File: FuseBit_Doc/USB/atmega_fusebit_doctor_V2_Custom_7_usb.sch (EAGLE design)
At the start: 73 parts, among them IC1 7805, IC10 MEGA8/88/168..., IC11 MEGA8-AI, IC12 FT232RL, IC14 TINY2313, IC15 MEGA16, IC16 MEGA128-A, IC17 MEGA8/88/168..., IC2 ATMEGA8-DOC, IC3 MEGA16/32/644..., IC4 MEGA8/88/168..., IC5 AT90S2313/TINY2313, IC8 AT90S8515PDIL40_OCT, IC9 TINY26, T1 BC857, T2 BC847, T3 BC557

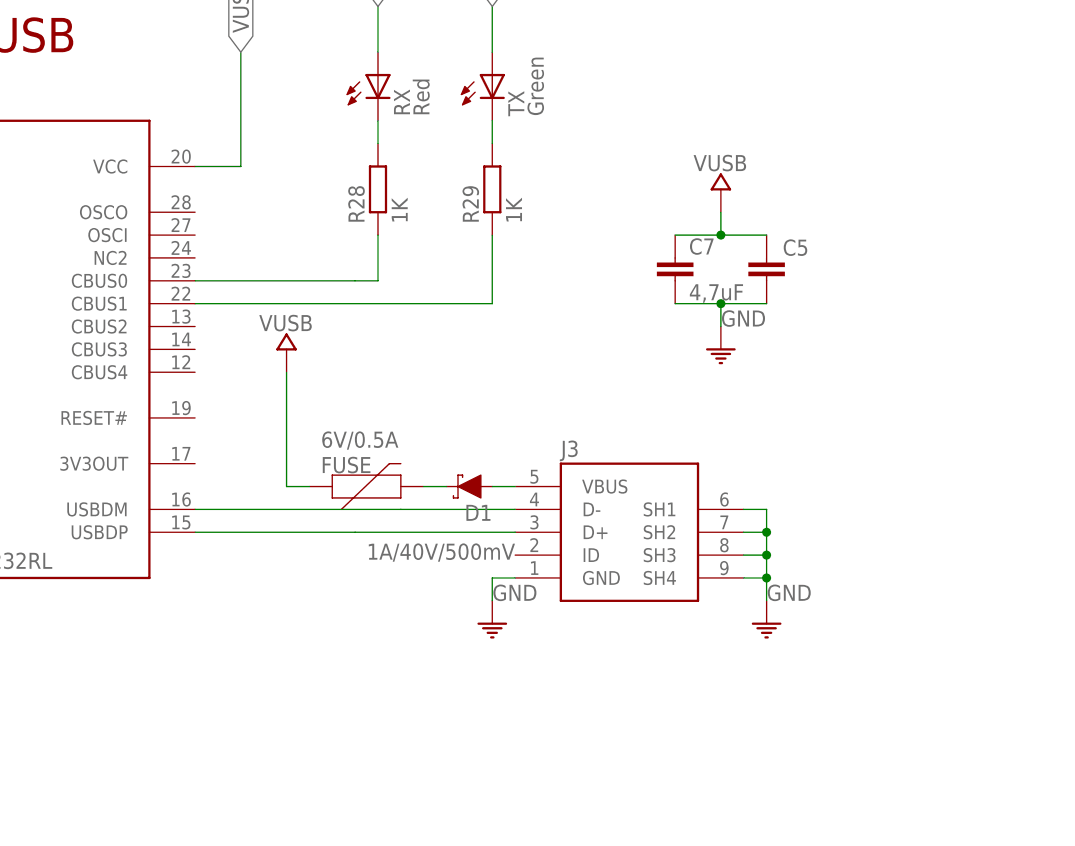
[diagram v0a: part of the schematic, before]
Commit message: FT232_update
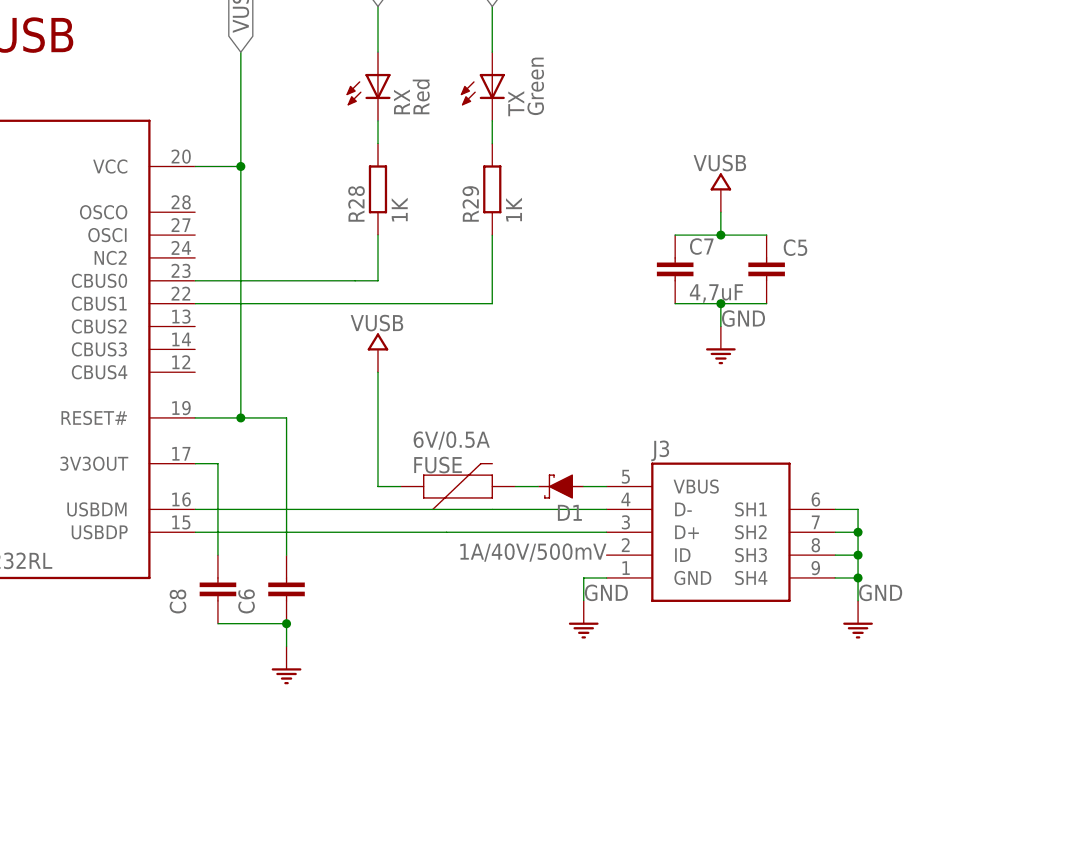
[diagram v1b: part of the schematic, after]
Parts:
- added C6, C8: 100nF, resistor@1:C-EUC0805
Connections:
- new net COM: C6.1, C8.1
- new net N$3: C8.2, IC12.3V3OUT
- net VUSB: now also C6.2, IC12.RESET#
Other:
- moved on the sheet: D1, FUSE, J3
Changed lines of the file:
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@@
 <?xml version="1.0" encoding="utf-8"?>
 <!DOCTYPE eagle SYSTEM "eagle.dtd">
-<eagle version="7.6.0">
+<eagle version="8.5.1">
 <drawing>
 <settings>
 <setting alwaysvectorfont="no"/>
+<setting keepoldvectorfont="yes"/>
 <setting verticaltext="up"/>
 </settings>
@@
 <part name="U$4" library="MyPOW" deviceset="VUSB" device=""/>
 <part name="D1" library="SparkFun-DiscreteSemi" deviceset="DIODE-SCHOTTKY" device="-SS14" value="1A/40V/500mV"/>
+<part name="C6" library="resistor@1" deviceset="C-EU" device="C0805" value="100nF"/>
+<part name="U$1" library="MyPOW" deviceset="COM" device=""/>
+<part name="C8" library="resistor@1" deviceset="C-EU" device="C0805" value="100nF"/>
 </parts>
 <sheets>
@@
 </instance>
 <instance part="U$24" gate="G$1" x="302.26" y="193.04"/>
-<instance part="U$22" gate="G$1" x="350.52" y="220.98"/>
-<instance part="U$29" gate="G$1" x="373.38" y="190.5"/>
-<instance part="U$30" gate="G$1" x="403.86" y="190.5"/>
-<instance part="J3" gate="G$1" x="388.62" y="200.66"/>
+<instance part="U$22" gate="G$1" x="360.68" y="220.98"/>
+<instance part="U$29" gate="G$1" x="383.54" y="190.5"/>
+<instance part="U$30" gate="G$1" x="414.02" y="190.5"/>
+<instance part="J3" gate="G$1" x="398.78" y="200.66"/>
 <instance part="U$51" gate="G$1" x="289.56" y="203.2"/>
 <instance part="RX" gate="G$1" x="360.68" y="251.46"/>
 <instance part="TX" gate="G$1" x="373.38" y="251.46"/>
 <instance part="IC12" gate="G$1" x="322.58" y="220.98"/>
-<instance part="FUSE" gate="G$1" x="358.14" y="205.74" smashed="yes">
-<attribute name="NAME" x="354.33" y="207.2386" size="1.778" layer="95"/>
-<attribute name="VALUE" x="354.33" y="210.058" size="1.778" layer="96"/>
+<instance part="FUSE" gate="G$1" x="368.3" y="205.74" smashed="yes">
+<attribute name="NAME" x="364.49" y="207.2386" size="1.778" layer="95"/>
+<attribute name="VALUE" x="364.49" y="210.058" size="1.778" layer="96"/>
 </instance>
 <instance part="R28" gate="G$1" x="360.68" y="238.76" rot="R90"/>
@@
 <instance part="C7" gate="G$1" x="393.7" y="231.14"/>
 <instance part="U$4" gate="G$1" x="398.78" y="238.76"/>
-<instance part="D1" gate="G$1" x="370.84" y="205.74" smashed="yes" rot="R180">
-<attribute name="NAME" x="373.38" y="203.708" size="1.778" layer="95" font="vector" rot="R180"/>
-<attribute name="VALUE" x="375.92" y="197.612" size="1.778" layer="96" font="vector" rot="R180" align="top-left"/>
+<instance part="D1" gate="G$1" x="381" y="205.74" smashed="yes" rot="R180">
+<attribute name="NAME" x="383.54" y="203.708" size="1.778" layer="95" font="vector" rot="R180"/>
+<attribute name="VALUE" x="386.08" y="197.612" size="1.778" layer="96" font="vector" rot="R180" align="top-left"/>
+</instance>
+<instance part="C6" gate="G$1" x="350.52" y="193.04" smashed="yes" rot="R180">
+<attribute name="NAME" x="346.964" y="191.516" size="1.778" layer="95" rot="R90"/>
+</instance>
+<instance part="U$1" gate="G$1" x="350.52" y="185.42"/>
+<instance part="C8" gate="G$1" x="342.9" y="193.04" smashed="yes" rot="R180">
+<attribute name="NAME" x="339.344" y="191.516" size="1.778" layer="95" rot="R90"/>
 </instance>
 </instances>
@@
 </segment>
 <segment>
-<wire x1="375.92" y1="195.58" x2="373.38" y2="195.58" width="0.1524" layer="91"/>
-<wire x1="373.38" y1="195.58" x2="373.38" y2="193.04" width="0.1524" layer="91"/>
+<wire x1="386.08" y1="195.58" x2="383.54" y2="195.58" width="0.1524" layer="91"/>
+<wire x1="383.54" y1="195.58" x2="383.54" y2="193.04" width="0.1524" layer="91"/>
 <pinref part="U$29" gate="G$1" pin="COM"/>
 <pinref part="J3" gate="G$1" pin="GND"/>
-<label x="373.38" y="193.04" size="1.778" layer="95"/>
+<label x="383.54" y="193.04" size="1.778" layer="95"/>
 </segment>
 <segment>
-<wire x1="403.86" y1="203.2" x2="403.86" y2="200.66" width="0.1524" layer="91"/>
-<wire x1="403.86" y1="200.66" x2="403.86" y2="198.12" width="0.1524" layer="91"/>
-<wire x1="403.86" y1="198.12" x2="403.86" y2="195.58" width="0.1524" layer="91"/>
-<wire x1="403.86" y1="195.58" x2="403.86" y2="193.04" width="0.1524" layer="91"/>
-<wire x1="401.32" y1="200.66" x2="403.86" y2="200.66" width="0.1524" layer="91"/>
-<wire x1="401.32" y1="195.58" x2="403.86" y2="195.58" width="0.1524" layer="91"/>
-<wire x1="401.32" y1="198.12" x2="403.86" y2="198.12" width="0.1524" layer="91"/>
-<wire x1="401.32" y1="203.2" x2="403.86" y2="203.2" width="0.1524" layer="91"/>
+<wire x1="414.02" y1="203.2" x2="414.02" y2="200.66" width="0.1524" layer="91"/>
+<wire x1="414.02" y1="200.66" x2="414.02" y2="198.12" width="0.1524" layer="91"/>
+<wire x1="414.02" y1="198.12" x2="414.02" y2="195.58" width="0.1524" layer="91"/>
+<wire x1="414.02" y1="195.58" x2="414.02" y2="193.04" width="0.1524" layer="91"/>
+<wire x1="411.48" y1="200.66" x2="414.02" y2="200.66" width="0.1524" layer="91"/>
+<wire x1="411.48" y1="195.58" x2="414.02" y2="195.58" width="0.1524" layer="91"/>
+<wire x1="411.48" y1="198.12" x2="414.02" y2="198.12" width="0.1524" layer="91"/>
+<wire x1="411.48" y1="203.2" x2="414.02" y2="203.2" width="0.1524" layer="91"/>
 <pinref part="U$30" gate="G$1" pin="COM"/>
 <pinref part="J3" gate="G$1" pin="SH2"/>
@@
 <pinref part="J3" gate="G$1" pin="SH3"/>
 <pinref part="J3" gate="G$1" pin="SH1"/>
-<junction x="403.86" y="200.66"/>
-<junction x="403.86" y="198.12"/>
-<junction x="403.86" y="195.58"/>
-<label x="403.86" y="193.04" size="1.778" layer="95"/>
+<junction x="414.02" y="200.66"/>
+<junction x="414.02" y="198.12"/>
+<junction x="414.02" y="195.58"/>
+<label x="414.02" y="193.04" size="1.778" layer="95"/>
 </segment>
 <segment>
@@
 <net name="VUSB" class="1">
 <segment>
-<wire x1="350.52" y1="205.74" x2="350.52" y2="218.44" width="0.1524" layer="91"/>
+<wire x1="360.68" y1="205.74" x2="360.68" y2="218.44" width="0.1524" layer="91"/>
 <pinref part="U$22" gate="G$1" pin="VUSB"/>
 <pinref part="FUSE" gate="G$1" pin="1"/>
-<wire x1="350.52" y1="205.74" x2="353.06" y2="205.74" width="0.1524" layer="91"/>
+<wire x1="360.68" y1="205.74" x2="363.22" y2="205.74" width="0.1524" layer="91"/>
 </segment>
 <segment>
@@
 <wire x1="345.44" y1="241.3" x2="345.44" y2="254" width="0.1524" layer="91"/>
 <label x="345.44" y="254" size="1.778" layer="95" rot="R90" xref="yes"/>
+<wire x1="345.44" y1="241.3" x2="345.44" y2="213.36" width="0.1524" layer="91"/>
+<junction x="345.44" y="241.3"/>
+<pinref part="IC12" gate="G$1" pin="RESET#"/>
+<wire x1="345.44" y1="213.36" x2="340.36" y2="213.36" width="0.1524" layer="91"/>
+<pinref part="C6" gate="G$1" pin="2"/>
+<wire x1="345.44" y1="213.36" x2="350.52" y2="213.36" width="0.1524" layer="91"/>
+<wire x1="350.52" y1="213.36" x2="350.52" y2="198.12" width="0.1524" layer="91"/>
+<junction x="345.44" y="213.36"/>
 </segment>
 <segment>
@@
 <net name="N$44" class="0">
 <segment>
-<wire x1="340.36" y1="200.66" x2="358.14" y2="200.66" width="0.1524" layer="91"/>
+<wire x1="340.36" y1="200.66" x2="368.3" y2="200.66" width="0.1524" layer="91"/>
 <pinref part="J3" gate="G$1" pin="D+"/>
 <pinref part="IC12" gate="G$1" pin="USBDP"/>
-<wire x1="358.14" y1="200.66" x2="375.92" y2="200.66" width="0.1524" layer="91"/>
+<wire x1="368.3" y1="200.66" x2="386.08" y2="200.66" width="0.1524" layer="91"/>
 </segment>
 </net>
 <net name="N$45" class="0">
 <segment>
-<wire x1="340.36" y1="203.2" x2="363.22" y2="203.2" width="0.1524" layer="91"/>
+<wire x1="340.36" y1="203.2" x2="373.38" y2="203.2" width="0.1524" layer="91"/>
 <pinref part="J3" gate="G$1" pin="D-"/>
 <pinref part="IC12" gate="G$1" pin="USBDM"/>
-<wire x1="363.22" y1="203.2" x2="375.92" y2="203.2" width="0.1524" layer="91"/>
+<wire x1="373.38" y1="203.2" x2="386.08" y2="203.2" width="0.1524" layer="91"/>
 </segment>
 </net>
@@
 <pinref part="FUSE" gate="G$1" pin="2"/>
 <pinref part="D1" gate="G$1" pin="C"/>
-<wire x1="365.76" y1="205.74" x2="368.3" y2="205.74" width="0.1524" layer="91"/>
+<wire x1="375.92" y1="205.74" x2="378.46" y2="205.74" width="0.1524" layer="91"/>
 </segment>
 </net>
@@
 <pinref part="D1" gate="G$1" pin="A"/>
 <pinref part="J3" gate="G$1" pin="VBUS"/>
-<wire x1="373.38" y1="205.74" x2="375.92" y2="205.74" width="0.1524" layer="91"/>
+<wire x1="383.54" y1="205.74" x2="386.08" y2="205.74" width="0.1524" layer="91"/>
+</segment>
+</net>
+<net name="COM" class="0">
+<segment>
+<pinref part="U$1" gate="G$1" pin="COM"/>
+<pinref part="C6" gate="G$1" pin="1"/>
+<wire x1="350.52" y1="187.96" x2="350.52" y2="190.5" width="0.1524" layer="91"/>
+<pinref part="C8" gate="G$1" pin="1"/>
+<wire x1="342.9" y1="190.5" x2="350.52" y2="190.5" width="0.1524" layer="91"/>
+<junction x="350.52" y="190.5"/>
+</segment>
+</net>
+<net name="N$3" class="0">
+<segment>
+<pinref part="IC12" gate="G$1" pin="3V3OUT"/>
+<wire x1="340.36" y1="208.28" x2="342.9" y2="208.28" width="0.1524" layer="91"/>
+<pinref part="C8" gate="G$1" pin="2"/>
+<wire x1="342.9" y1="208.28" x2="342.9" y2="198.12" width="0.1524" layer="91"/>
 </segment>
 </net>
